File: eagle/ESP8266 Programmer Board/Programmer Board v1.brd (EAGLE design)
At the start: 160 x 100 mm, 11 parts, among them J1 FTDI, J2 DCJ0202, U1 LM7833

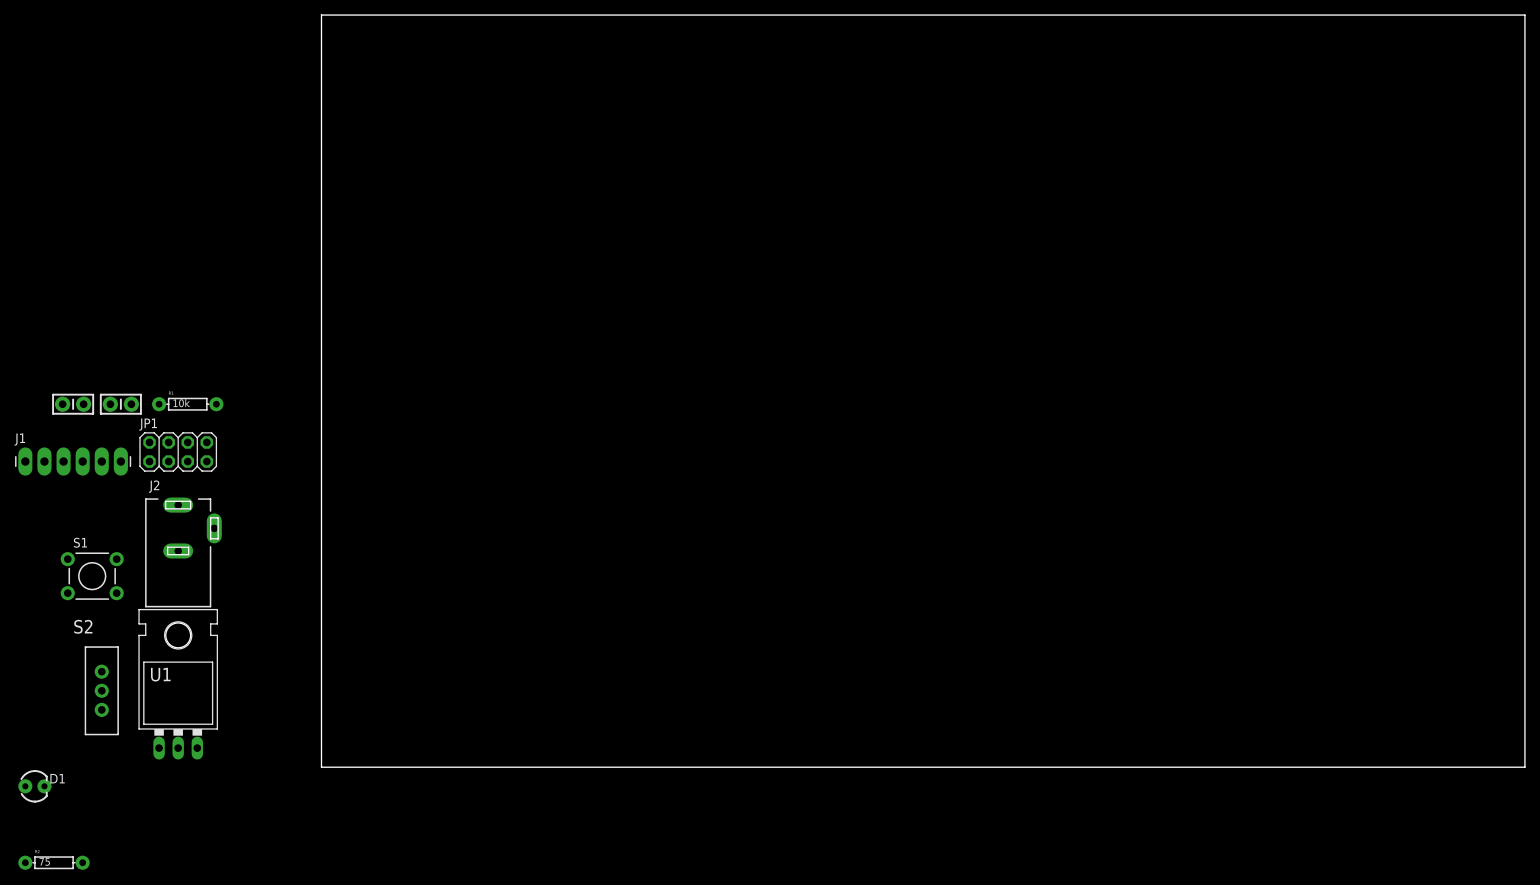
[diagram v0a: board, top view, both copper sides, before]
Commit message: Updating switches
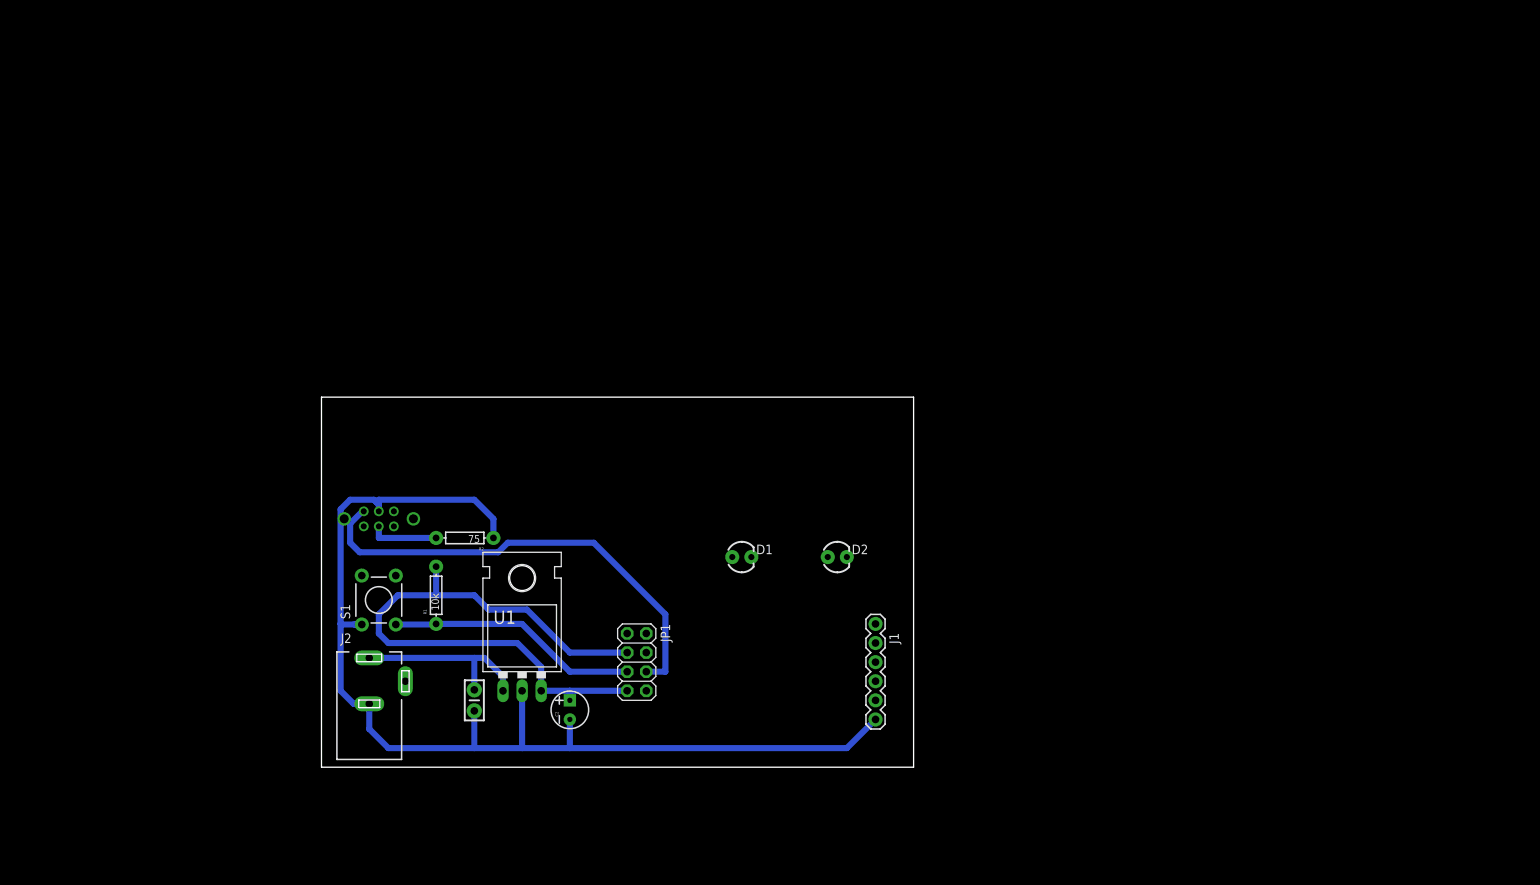
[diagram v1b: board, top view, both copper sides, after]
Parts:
- added D2: PROG, SparkFun-LED:LED3MM
- C1: value (none) -> 0.1uF
- C2: value (none) -> 10uF; device SparkFun-Capacitors:CAP-PTH-SMALL-KIT -> SparkFun-Capacitors:CPOL-RADIAL-10UF-25V-KIT
- J1: device SparkFun-Connectors:1X06_LONGPADS -> SparkFun-Connectors:FTDI_BASIC
- S2: value PROG -> (none); device SparkFun-Electromechanical:SWITCH-SPDT -> SparkFun-Electromechanical:EG2211
- moved J1 115.1 mm to (73.7, 19.1), turned to 270 degrees
- moved D1 98.8 mm to (55.9, 27.9)
- moved C2 77.5 mm to (33.0, 7.62), turned to 90 degrees
- moved R2 69.6 mm to (19.1, 30.5), turned to 180 degrees
- moved JP1 67.1 mm to (41.9, 14.0), turned to 270 degrees
- moved C1 61.3 mm to (20.3, 8.89), turned to 270 degrees
- moved U1 46.4 mm to (26.7, 14.0)
- moved S2 43.3 mm to (7.62, 33.0), turned to 270 degrees
- moved R1 41.7 mm to (15.2, 22.9), turned to 90 degrees
- moved S1 38.2 mm to (7.62, 22.2), turned to 90 degrees
- moved J2 32.5 mm to (6.35, 11.4)
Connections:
- removed net 3V3: JP1.7
- removed net CH_PD: JP1.3, S2.3
- removed net N$1: D1.K, R2.P$2
- new net N$3: D1.K, S2.P2-TA
- new net N$4: R2.P$2, S2.P2
- net +3V3: now also D2.A, JP1.3, JP1.7
- net GND: now also J1.GND, R2.P$1, S2.P1; no longer J1.6, S2.2
- net GPIO0: now also S2.P1-TB
- net N$2: now also D2.K, S2.P2-TB; no longer R2.P$1, S2.1
- net RX: now also J1.TXO; no longer J1.3
- net TX: now also J1.RXI; no longer J1.2
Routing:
- net GND: track 0.00 -> 148.2 mm
- net +3V3: track 0.00 -> 82.9 mm
- net GPIO0: track 0.00 -> 62.1 mm
- net RST: track 0.00 -> 33.4 mm
- net VCC: track 0.00 -> 24.9 mm
- net N$4: track 0.00 -> 9.16 mm
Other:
- board size 160 x 100 mm -> 78.7 x 49.2 mm
